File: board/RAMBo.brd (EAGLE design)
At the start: 104.1 x 102.9 mm, 273 parts, among them Q1 PSMN7R0-60YS, Q2 PSMN7R0-60YS, Q3 PSMN7R0-60YS, Q4 IRLML6346TRPBF, Q5 PSMN7R0-60YS, Q8 IRLML6346TRPBF, U1 ATMEGA32U2-MUR, U10 ADUM7441, U2 ATMEGA2560-16AU, U3 TPS54332DDA, U4 AD5206, U5 A4982, U6 A4982, U7 A4982, U8 A4982, U9 A4982, X1 C-GRID-02-70543, X10 C-GRID-04-70543, X11 MSTBV10, X12 SPI, X13 EXT-2, X14 C-GRID-04-70543, X15 C-GRID-04-70543, X16 32u2 EXT, X17 3x2M, X18 3x2M, X2 USB B-TH, X20 M05PTH, X21 C-GRID-03-70543, X22 C-GRID-03-70543, X23 C-GRID-03-70543, X24 C-GRID-03-70543, X25 C-GRID-03-70543, X26 C-GRID-03-70543, X27 C-GRID-02-70543, X28 C-GRID-02-70543, X29 C-GRID-02-70543, X3 C-GRID-02-70543, X30 C-GRID-02-70543, X31 M05PTH, X32 M05PTH, X33 MSTBA6, X34 PWM_EXT, X39 M05X2PTH, X4 C-GRID-04-70543, X40 Analog, X5 C-GRID-02-70543, X6 C-GRID-04-70543, X7 C-GRID-04-70543, X8 C-GRID-04-70543, X9 C-GRID-02-70543, Y1 16MHz KX-7, Y2 16MHz KX-7

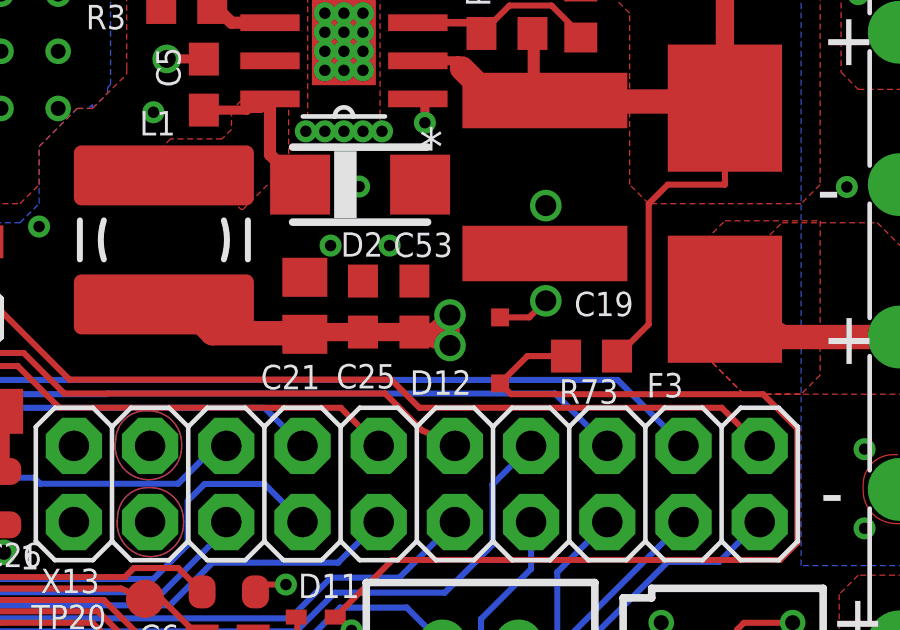
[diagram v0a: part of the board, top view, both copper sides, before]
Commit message: set L2 part
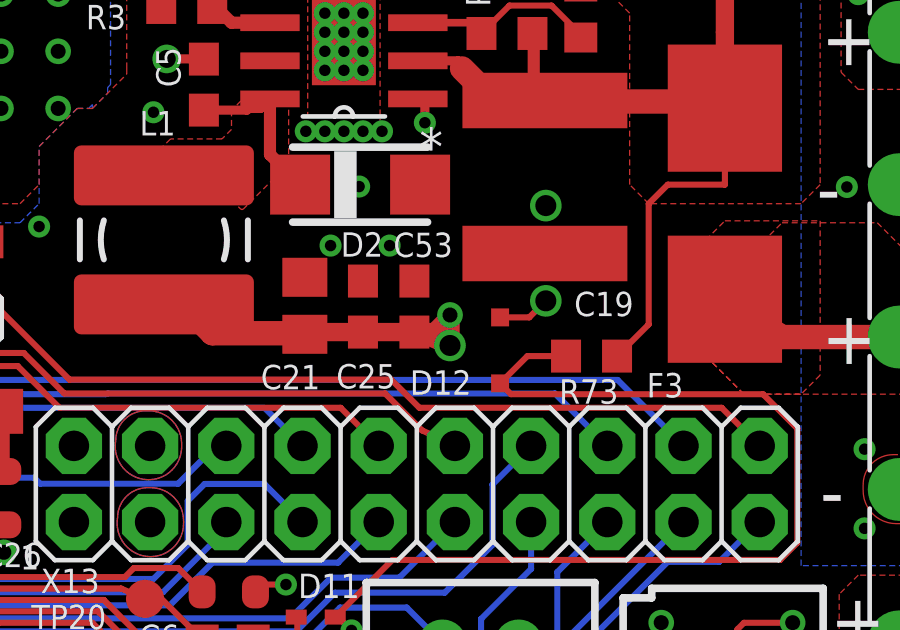
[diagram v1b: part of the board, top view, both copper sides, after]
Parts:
- D9: value S3A -> 1SMB5935BT3G
- L2: value (none) -> CBC2012T100M
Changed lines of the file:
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@@
 <attribute name="NAME" x="98.656" y="30.281" size="0.8128" layer="25" rot="R90"/>
 </element>
-<element name="D9" library="diode" package="SMB" value="S3A" x="88.646" y="86.36" smashed="yes" rot="R90">
+<element name="D9" library="diode" package="SMB" value="1SMB5935BT3G" x="88.646" y="86.36" smashed="yes" rot="R90">
 <attribute name="NAME" x="84.8025" y="90.22" size="0.8128" layer="25"/>
 </element>
@@
 <attribute name="VALUE" x="71.1835" y="50.9905" size="1.27" layer="27" rot="R90"/>
 </element>
-<element name="L2" library="resistor" package="C0805" value="" x="64.008" y="68.6435" smashed="yes">
+<element name="L2" library="resistor" package="C0805" value="CBC2012T100M" x="64.008" y="68.6435" smashed="yes">
 <attribute name="NAME" x="60.8965" y="67.8815" size="0.8128" layer="25"/>
 <attribute name="VALUE" x="63.119" y="66.3575" size="1.27" layer="27"/>
@@
 <wire x1="36.1315" y1="56.3635" x2="35.98" y2="56.515" width="0.2032" layer="1"/>
 <via x="79.73675" y="70.83875" extent="1-16" drill="0.7"/>
-<via x="79.73675" y="71.85475" extent="1-16" drill="0.7"/>
+<via x="79.73675" y="71.85475" extent="1-16" drill="0.5"/>
 <wire x1="78.5495" y1="71.286" x2="78.6545" y2="71.286" width="0.6096" layer="1"/>
 <wire x1="78.6545" y1="71.286" x2="79.73675" y2="70.83875" width="0.6096" layer="1"/>
